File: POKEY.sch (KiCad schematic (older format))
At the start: 64 parts, among them J108 pin, J109 pin, J110 pin, J111 pin, U22 POKEY, U24 CD4051B, U25 CD4051B

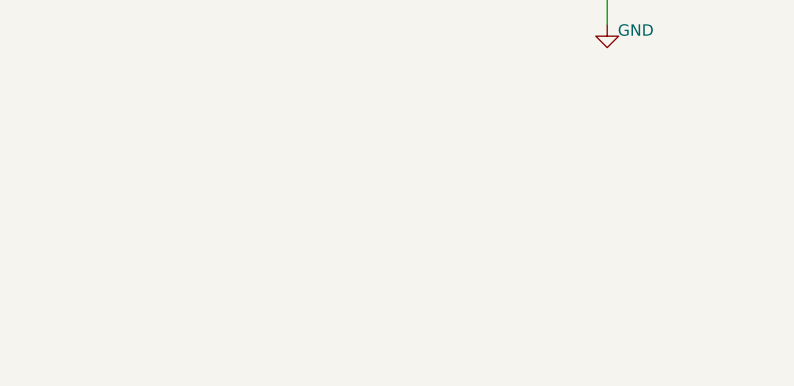
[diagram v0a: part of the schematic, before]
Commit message: Trackimg
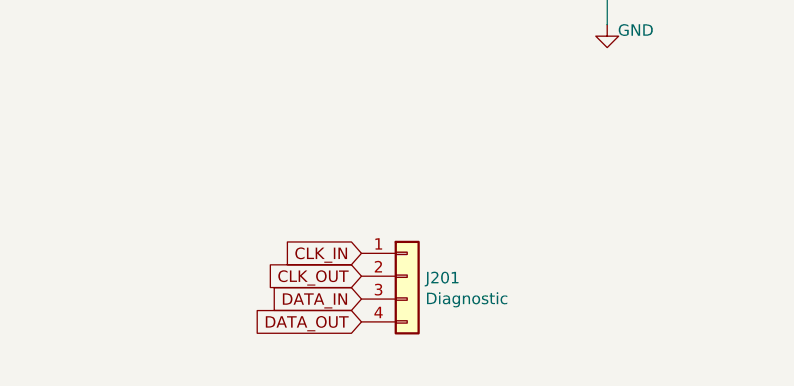
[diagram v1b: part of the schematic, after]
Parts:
- added J201: Diagnostic, Connector_PinHeader_2.54mm:PinHeader_1x04_P2.54mm_Vertical, symbol Connector_Generic:Conn_01x04
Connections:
- net CLK_IN: now also J201.1 (Pin_1)
- net CLK_OUT: now also J201.2 (Pin_2)
- net DATA_IN: now also J201.3 (Pin_3)
- net DATA_OUT: now also J201.4 (Pin_4)
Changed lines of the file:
@@
 	5950 5825 5950 5700
 Connection ~ 5950 5700
+$Comp
+L Connector_Generic:Conn_01x04 J201
+U 1 1 604341BE
+P 2425 6050
+F 0 "J201" H 2505 6042 50  0000 L CNN
+F 1 "Diagnostic" H 2505 5951 50  0000 L CNN
+F 2 "Connector_PinHeader_2.54mm:PinHeader_1x04_P2.54mm_Vertical" H 2425 6050 50  0001 C CNN
+F 3 "~" H 2425 6050 50  0001 C CNN
+	1    2425 6050
+	1    0    0    -1
+$EndComp
+Text GLabel 2225 6050 0    50   Input ~ 0
+CLK_OUT
+Text GLabel 2225 5950 0    50   Input ~ 0
+CLK_IN
+Text GLabel 2225 6150 0    50   Input ~ 0
+DATA_IN
+Text GLabel 2225 6250 0    50   Input ~ 0
+DATA_OUT
 $EndSCHEMATC
